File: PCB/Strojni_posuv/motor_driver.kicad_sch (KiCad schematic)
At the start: 50 parts, among them IC1 TB6600HG, J3 OUT1, J4 OUT2, Q1 BSS138, Q2 BSS138, Q3 BSS138, Q4 BSS138, Q5 BSS138, Q6 BSS138, Q7 BC847, U7 74HC14

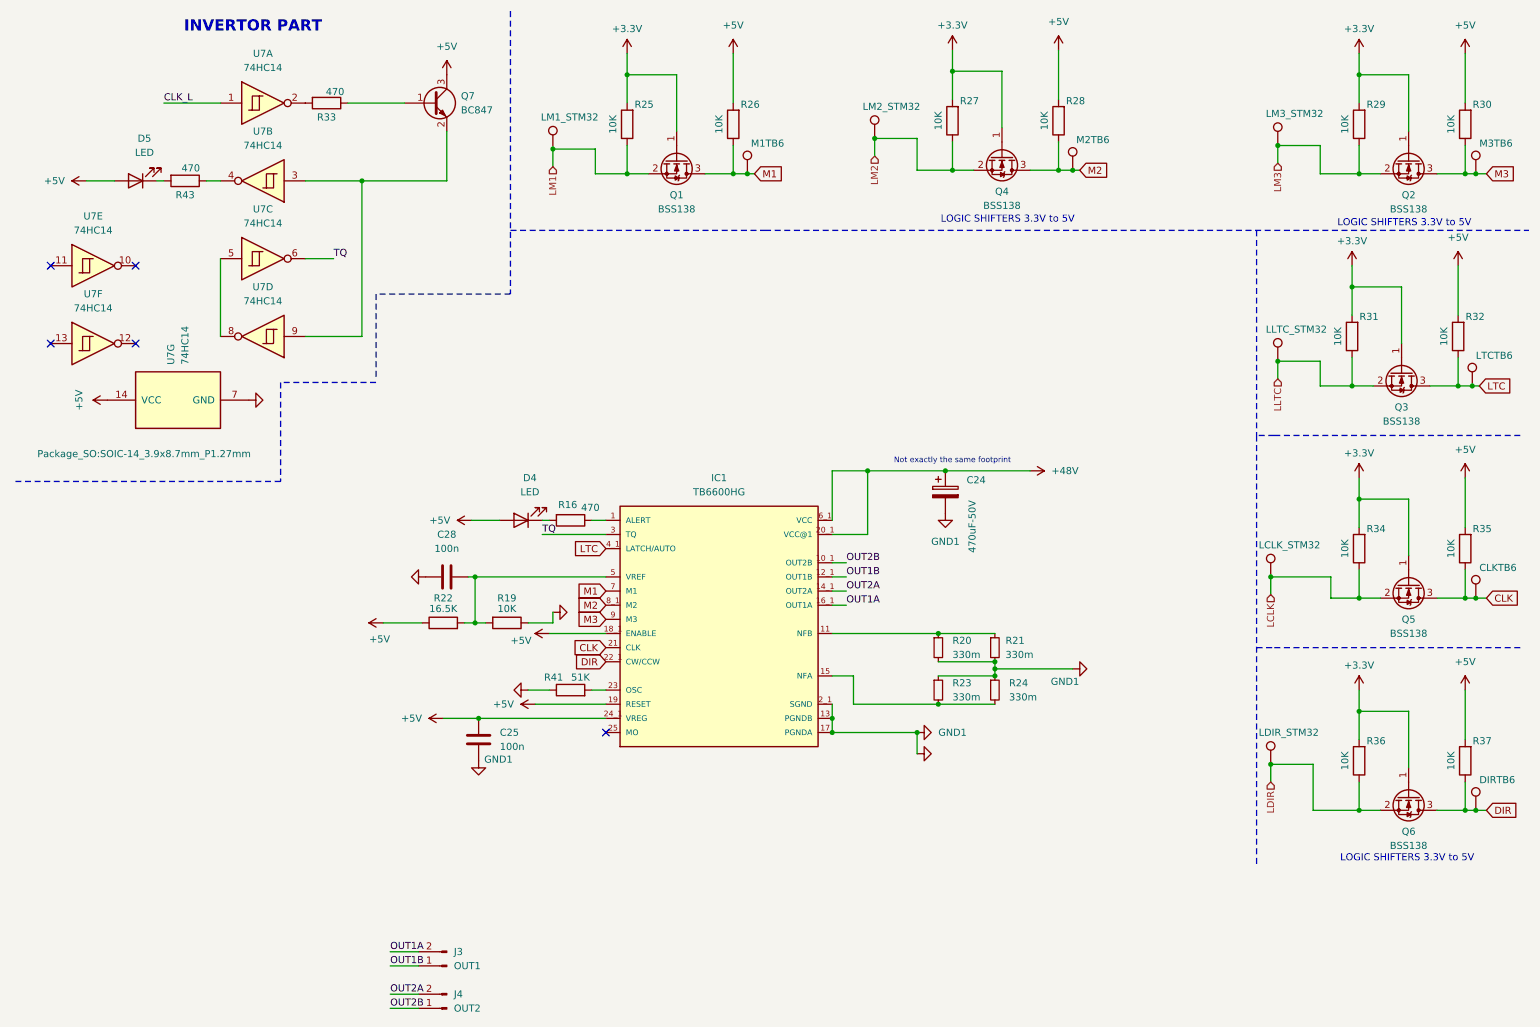
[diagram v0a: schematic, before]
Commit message: Schema done?
I think that I have functional schema, but it needs a check
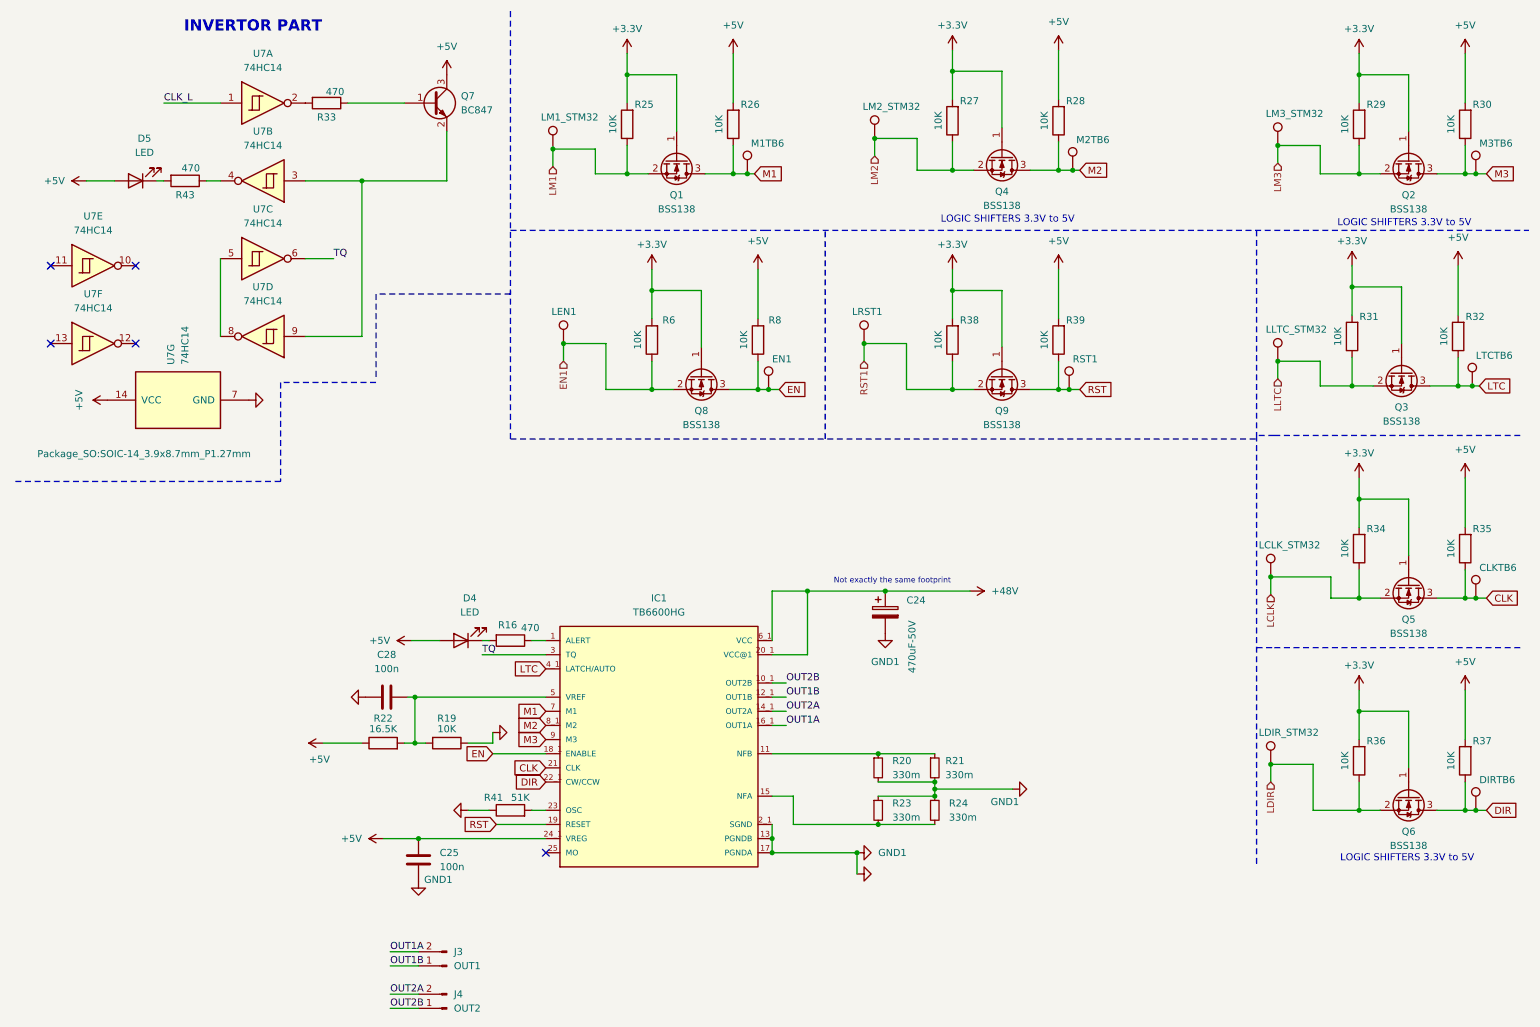
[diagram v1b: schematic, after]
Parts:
- added EN1, LEN1, LRST1, RST1: ~, TestPoint:TestPoint_Pad_D1.0mm, symbol Connector:TestPoint
- added Q8, Q9: BSS138, Package_TO_SOT_SMD:SOT-23, symbol Transistor_FET:BSS138
- added R38, R39, R6, R8: 10K, Resistor_SMD:R_0805_2012Metric, symbol Device:R
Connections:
- net +3.3V: now also Q8.1 (G), Q9.1 (G), R38.2, R6.2
- net +5V: now also R39.2, R8.2; no longer IC1.18_1 (ENABLE), IC1.19 (RESET)
- new net EN: EN1.1, IC1.18_1 (ENABLE), Q8.3 (D), R8.1
- new net EN1: LEN1.1, Q8.2 (S), R6.1
- new net RST: IC1.19 (RESET), Q9.3 (D), R39.1, RST1.1
- new net RST1: LRST1.1, Q9.2 (S), R38.1
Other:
- moved on the sheet: C24, C25, C28, D4, IC1, R16, R19, R20, R21, R22, R23, R24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

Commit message: PCB done?
I did all the routing and component placement on PCB
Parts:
- J3, J4: footprint Connector_PinSocket_2.54mm:PinSocket_1x02_P2.54mm_Vertical -> TerminalBlock_Phoenix:TerminalBlock_Phoenix_MKDS-1,5-2-5.08_1x02_P5.08mm_Horizontal
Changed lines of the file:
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@@
 			)
 		)
-		(property "Footprint" "Connector_PinSocket_2.54mm:PinSocket_1x02_P2.54mm_Vertical"
+		(property "Footprint" "TerminalBlock_Phoenix:TerminalBlock_Phoenix_MKDS-1,5-2-5.08_1x02_P5.08mm_Horizontal"
 			(at 90.17 184.15 0)
 			(effects
@@
 			)
 		)
-		(property "Footprint" "Connector_PinSocket_2.54mm:PinSocket_1x02_P2.54mm_Vertical"
+		(property "Footprint" "TerminalBlock_Phoenix:TerminalBlock_Phoenix_MKDS-1,5-2-5.08_1x02_P5.08mm_Horizontal"
 			(at 90.17 191.77 0)
 			(effects
